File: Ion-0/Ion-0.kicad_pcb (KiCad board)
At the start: 4 copper layers, 54.6 x 97.2 mm, 104 parts, among them J1 Beaglebone-green-P9, J10 Conn_Heater, J11 Conn_01x02, J12 Conn_01x02, J13 Conn_01x04, J2 Beaglebone-green-P8, J3 Conn_02x06_Odd_Even, J4 Conn_02x06_Odd_Even, J5 Conn_02x06_Odd_Even, J6 Coaxial_Small, J7 Conn_01x02, J8 Conn_Heater, J9 Conn_Heater, Q1 IRLML6244, Q2 IRLML6244, Q3 IRLML6244, Q4 IRLML6244, U2 LMT84DCK, U3 BNO085, U4 TCA9617ADGKR, U5 LMT84DCK, U6 MAX-M10M-00B, U7 TPS3850H50DRCR, U8 SN65HVD230, U9 MS860702BA01-50, Y2 9HT10-32.768KBZF-T

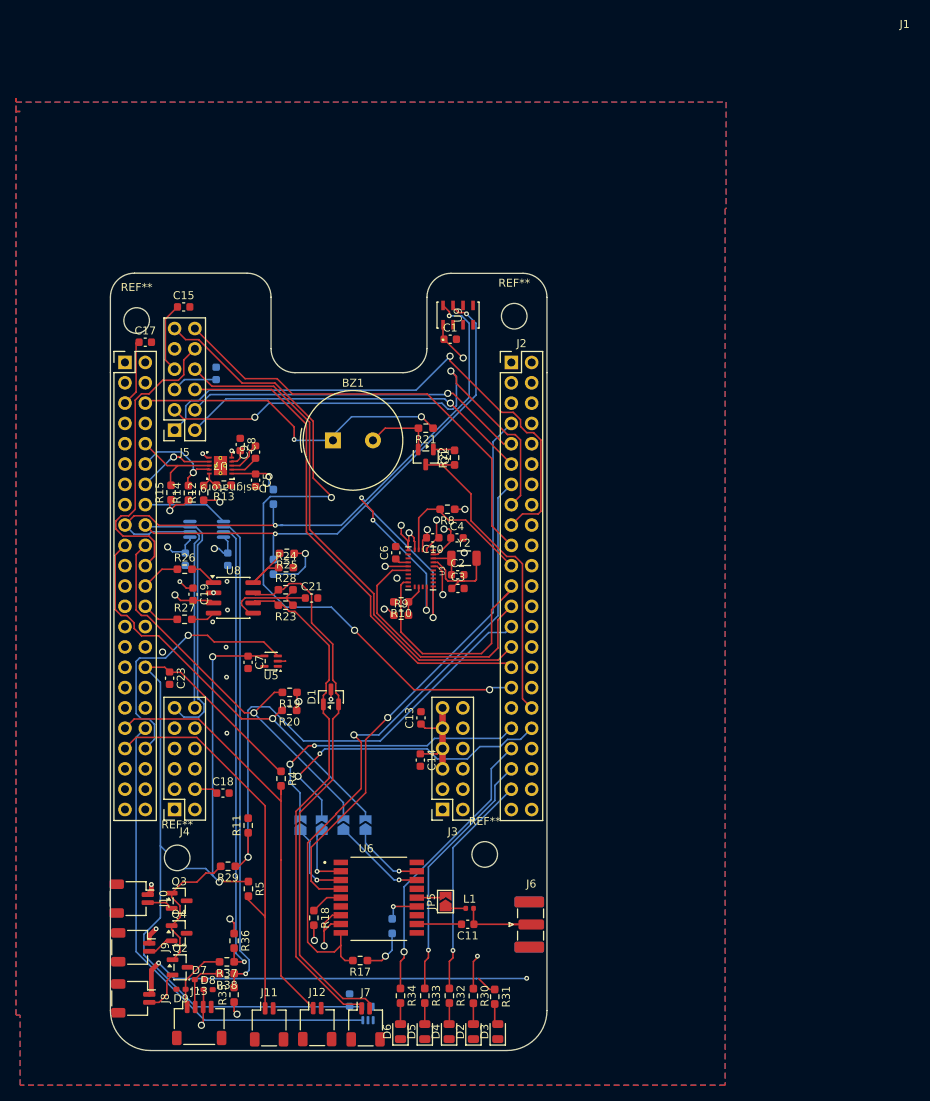
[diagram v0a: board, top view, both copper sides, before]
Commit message: restarting layout
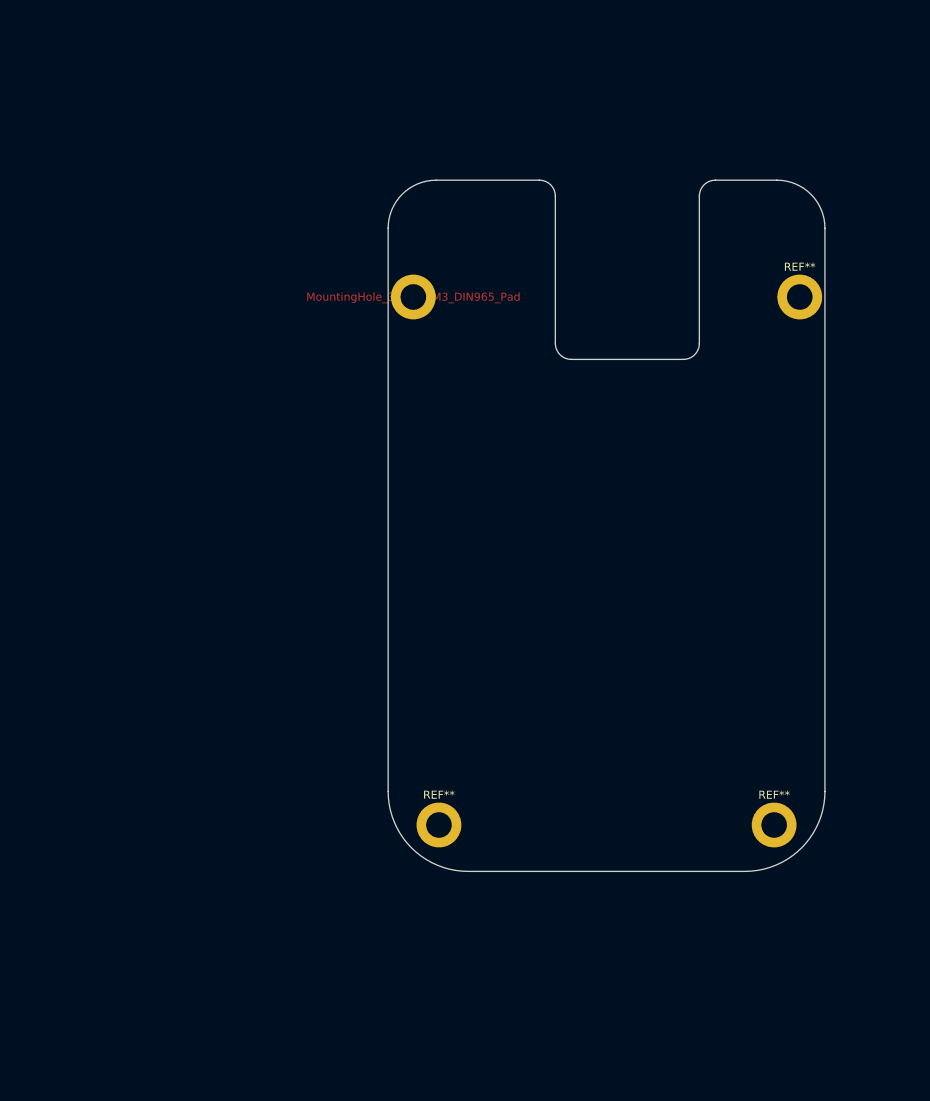
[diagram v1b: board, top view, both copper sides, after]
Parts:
- removed BZ1: PS1240P02BT, Buzzer_Beeper:Buzzer_TDK_PS1240P02BT_D12.2mm_H6.5mm
- removed C1: 220nF, Capacitor_SMD:C_0603_1608Metric
- removed C10, C12, C13, C15, C18, C19, C20: 100nF, Capacitor_SMD:C_0603_1608Metric
- removed C11: 47pF, Capacitor_SMD:C_0603_1608Metric
- removed C14, C16, C17: 22uF, Capacitor_SMD:C_0603_1608Metric
- removed C2, C3: 22pF, Capacitor_SMD:C_0603_1608Metric
- removed C21: 4.7nF, Capacitor_SMD:C_0603_1608Metric
- removed C22, C23, C7, C8: 1uF, Capacitor_SMD:C_0603_1608Metric
- removed C4, C5, C6: 0.1uF, Capacitor_SMD:C_0603_1608Metric
- removed C9: 100pF, Capacitor_SMD:C_0603_1608Metric
- removed D1: ESD3V3T2BHE3, Package_TO_SOT_SMD:SOT-23
- removed D2, D3, D4, D5, D6: LED, LED_SMD:LED_0805_2012Metric
- removed D7, D8, D9: TVS_3V3, Diode_SMD:D_0402_1005Metric_Pad0.77x0.64mm_HandSolder
- removed J1: Beaglebone-green-P9, Connector_PinHeader_2.54mm:PinHeader_2x23_P2.54mm_Vertical
- removed J10, J8, J9: Conn_Heater, Connector_JST:JST_SH_SM02B-SRSS-TB_1x02-1MP_P1.00mm_Horizontal
- removed J11, J12, J7: Conn_01x02, Connector_JST:JST_SH_SM02B-SRSS-TB_1x02-1MP_P1.00mm_Horizontal
- removed J13: Conn_01x04, Connector_JST:JST_SH_SM04B-SRSS-TB_1x04-1MP_P1.00mm_Horizontal
- removed J2: Beaglebone-green-P8, Connector_PinHeader_2.54mm:PinHeader_2x23_P2.54mm_Vertical
- removed J3, J4, J5: Conn_02x06_Odd_Even, Connector_PinSocket_2.54mm:PinSocket_2x06_P2.54mm_Vertical
- removed J6: Coaxial_Small, Connector_Coaxial:SMA_Samtec_SMA-J-P-H-ST-EM1_EdgeMount
- removed JP1, JP2, JP3, JP4, JP5: SolderJumper_2_Open, Jumper:SolderJumper-2_P1.3mm_Open_TrianglePad1.0x1.5mm
- removed L1: 101nH, Inductor_SMD:L_0402_1005Metric
- removed Q1, Q2, Q3, Q4: IRLML6244, Package_TO_SOT_SMD:SOT-23
- removed R10, R24: 0, Resistor_SMD:R_0603_1608Metric_Pad0.98x0.95mm_HandSolder
- removed R11, R14, R15, R16, R17, R35, R36, R8: 10K, Resistor_SMD:R_0603_1608Metric_Pad0.98x0.95mm_HandSolder
- removed R12: 523, Resistor_SMD:R_0603_1608Metric_Pad0.98x0.95mm_HandSolder
- removed R13: 80.6, Resistor_SMD:R_0603_1608Metric_Pad0.98x0.95mm_HandSolder
- removed R18, R19, R20, R6, R7: 4.7K, Resistor_SMD:R_0603_1608Metric_Pad0.98x0.95mm_HandSolder
- removed R21, R22, R29, R32, R33, R34, R37, R38: 330, Resistor_SMD:R_0603_1608Metric_Pad0.98x0.95mm_HandSolder
- removed R23, R28: 60, Resistor_SMD:R_0603_1608Metric_Pad0.98x0.95mm_HandSolder
- removed R25, R9: DNI, Resistor_SMD:R_0603_1608Metric_Pad0.98x0.95mm_HandSolder
- removed R26, R27: 33, Resistor_SMD:R_0603_1608Metric_Pad0.98x0.95mm_HandSolder
- removed R30: 470, Resistor_SMD:R_0603_1608Metric_Pad0.98x0.95mm_HandSolder
- removed R31: 1k, Resistor_SMD:R_0603_1608Metric_Pad0.98x0.95mm_HandSolder
- removed R4, R5: 100K, Resistor_SMD:R_0603_1608Metric_Pad0.98x0.95mm_HandSolder
- removed the REF** at (89.8, 74.9)
- removed the REF** at (137.0, 74.4)
- removed the REF** at (133.3, 141.7)
- removed the REF** at (94.8, 142.1)
- removed U2, U5: LMT84DCK, Package_TO_SOT_SMD:SOT-353_SC-70-5
- removed U3: BNO085, 1_Ion:IC_BNO085
- removed U4: TCA9617ADGKR, 1_Ion:TCA9617A
- removed U6: MAX-M10M-00B, 1_Ion:XCVR_MAX-M10M-00B
- removed U7: TPS3850H50DRCR, 1_Ion:TPS3850
- removed U8: SN65HVD230, Package_SO:SOIC-8_3.9x4.9mm_P1.27mm
- removed U9: MS860702BA01-50, 1_Ion:MS860702BA01-50_TEC
- removed Y2: 9HT10-32.768KBZF-T, Inductor_SMD:L_1206_3216Metric
- added REF**: MountingHole_3.2mm_M3_DIN965_Pad, MountingHole:MountingHole_3.2mm_M3_DIN965_Pad, F.Cu at (124.3, 72.0)
- added REF**: MountingHole_3.2mm_M3_DIN965_Pad, MountingHole:MountingHole_3.2mm_M3_DIN965_Pad, F.Cu at (169.4, 138.0)
- added REF**: MountingHole_3.2mm_M3_DIN965_Pad, MountingHole:MountingHole_3.2mm_M3_DIN965_Pad, F.Cu at (127.5, 138.0)
- added REF**: MountingHole_3.2mm_M3_DIN965_Pad, MountingHole:MountingHole_3.2mm_M3_DIN965_Pad, F.Cu at (172.7, 72.0)
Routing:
- net +1V8: track 136.8 -> 0.00 mm, vias 2 -> 0
- net +5V: track 127.7 -> 0.00 mm, vias 6 -> 0
- net /I2C1_SDA: track 122.2 -> 0.00 mm, vias 3 -> 0
- net /I2C1_SCL: track 120.6 -> 0.00 mm, vias 5 -> 0
- net +3V3: track 112.3 -> 0.00 mm, vias 20 -> 0
- net /IND_3: track 88.2 -> 0.00 mm, vias 3 -> 0
- net /GPIO_69: track 80.0 -> 0.00 mm, vias 1 -> 0
- net /Timer4: track 71.7 -> 0.00 mm, vias 1 -> 0
- net /SERVO_2: track 69.1 -> 0.00 mm, vias 1 -> 0
- net /Sensor-bus-hat/CAN_P: track 68.9 -> 0.00 mm
- net /MOTOR_2_A: track 64.7 -> 0.00 mm
- net /Sensor-bus-hat/CAN_N: track 64.4 -> 0.00 mm
- net /GPIO_86: track 64.4 -> 0.00 mm, vias 1 -> 0
- net /MOTOR_2_B: track 63.3 -> 0.00 mm
- net /SERVO_1: track 63.0 -> 0.00 mm, vias 2 -> 0
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- removed copper zone on In2.Cu, net +3V3
- removed copper zone on In2.Cu, net +5V
- removed copper zone on B.Cu, net GND
- removed copper zone on F.Cu, net GND
- removed copper zone on In1.Cu, net GND
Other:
- board size 54.6 x 97.2 mm -> 54.6 x 86.4 mm
